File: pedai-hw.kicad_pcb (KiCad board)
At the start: 2 copper layers, 59 parts, among them IC1 CD4051BE, IC2 CD4051BE, IC3 CD4051BE, IC4 CD4051BE, IC5 CD4051BE, IC6 CD4051BE, J1 Conn_01x06, J10 Conn_01x06, J15 Spare_ADC, J16 left_connector_blackpill, J17 right_connector_blackpill, J3 I2S_module, J5 LCD1602a, J6 Conn_01x06, J7 Conn_01x06, J8 Conn_01x06, J9 Conn_01x06

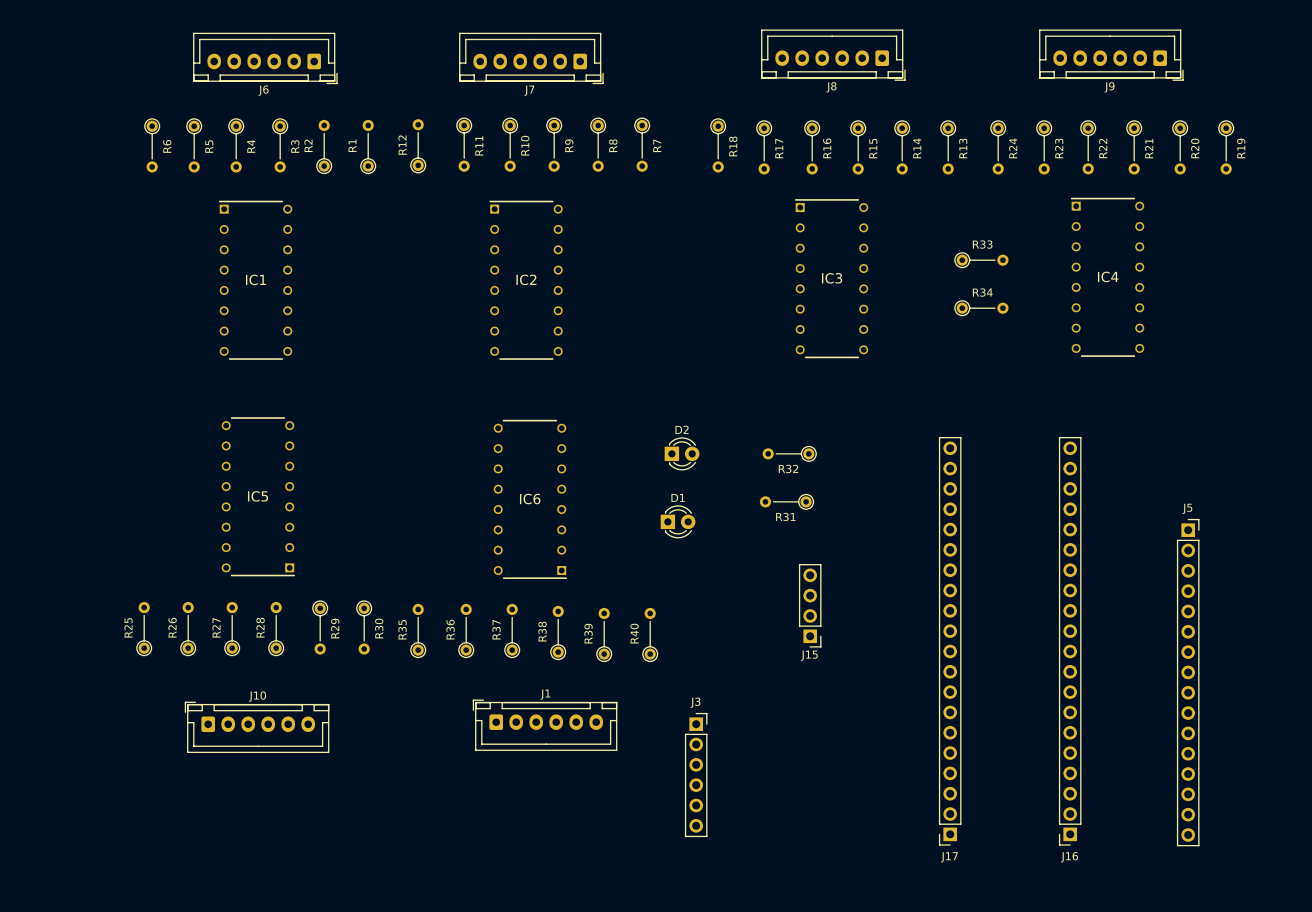
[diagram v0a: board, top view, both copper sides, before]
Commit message: layout and routing finished
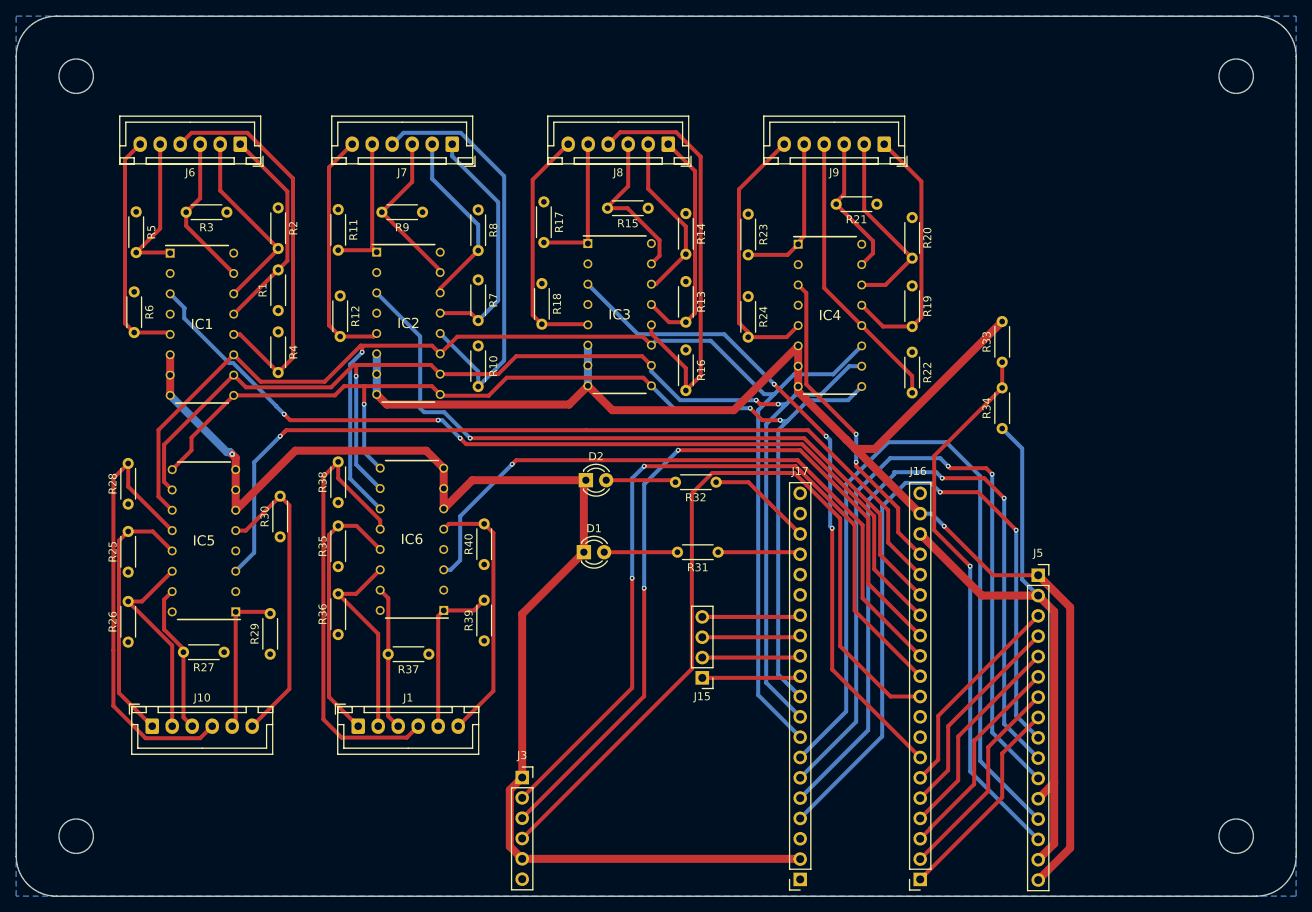
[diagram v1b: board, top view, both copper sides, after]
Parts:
- added H1: MountingHole, MountingHole:MountingHole_4.3mm_M4, F.Cu at (202.5, 32.5)
- added H2: MountingHole, MountingHole:MountingHole_4.3mm_M4, F.Cu at (202.5, 127.5)
- added H3: MountingHole, MountingHole:MountingHole_4.3mm_M4, F.Cu at (57.5, 32.5)
- added H4: MountingHole, MountingHole:MountingHole_4.3mm_M4, F.Cu at (57.5, 127.5)
- R1, R10, R11, R12, R13, R14, R15, R16, R17, R18, R19, R2, R20, R21, R22, R23, R24, R25, R26, R27, R28, R29, R3, R30, R31, R32, R33, R34, R35, R36, R37, R38, R39, R4, R40, R5, R6, R7, R8, R9: footprint Resistor_THT:R_Axial_DIN0204_L3.6mm_D1.6mm_P5.08mm_Vertical -> Resistor_THT:R_Axial_DIN0204_L3.6mm_D1.6mm_P5.08mm_Horizontal
- moved R19 43.9 mm to (162.0, 58.7)
- moved R23 38.5 mm to (141.5, 49.8)
- moved R13 38.0 mm to (133.7, 58.2)
- moved R24 37.7 mm to (141.5, 60.0)
- moved J9 36.1 mm to (158.5, 41.0)
- moved R22 35.6 mm to (162.0, 67.0)
- moved R20 35.3 mm to (162.0, 50.2)
- moved IC4 35.1 mm to (151.7, 62.4)
- moved R21 33.5 mm to (157.6, 48.5), turned to 180 degrees
- moved R38 33.3 mm to (90.2, 85.8)
- moved R16 31.9 mm to (133.7, 66.7)
- moved R18 29.5 mm to (115.7, 58.4)
- moved R14 29.1 mm to (133.7, 49.7)
- moved R17 29.0 mm to (116.0, 48.2)
- moved J8 28.8 mm to (131.5, 41.0)
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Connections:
- J17 pad 1: +5V -> unconnected-(J17-Pin_1-Pad1)
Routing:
- net GND: track 0.00 -> 344.6 mm, vias 0 -> 2
- net /MUX_C0: track 0.00 -> 181.6 mm, vias 0 -> 1
- net /MUX_C1: track 0.00 -> 163.5 mm, vias 0 -> 3
- net /MUX_C2: track 0.00 -> 144.2 mm, vias 0 -> 3
- net /MUX1_DATA: track 0.00 -> 115.1 mm, vias 0 -> 3
- net /MUX5_DATA: track 0.00 -> 109.5 mm, vias 0 -> 1
- net /LCD_RS: track 0.00 -> 103.1 mm
- net /I2S_WS: track 0.00 -> 102.4 mm
- net /I2S_CLK: track 0.00 -> 99.4 mm, vias 0 -> 2
- net /I2S_SD: track 0.00 -> 98.7 mm, vias 0 -> 2
- net /LCD_ENABLE: track 0.00 -> 98.6 mm, vias 0 -> 2
- net /LCD_D0: track 0.00 -> 95.0 mm, vias 0 -> 2
- net /MUX2_DATA: track 0.00 -> 91.8 mm, vias 0 -> 1
- net /LCD_D1: track 0.00 -> 90.8 mm, vias 0 -> 2
- net /MUX6_DATA: track 0.00 -> 83.9 mm, vias 0 -> 1
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- added copper zone on B.Cu, net +3.3V
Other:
- board outline added: 160 x 110 mm
